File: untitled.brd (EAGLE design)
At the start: 100 x 60 mm, 43 parts, among them J1 61300311121, Q1 FQPF10N60C, Q2 s8550, Q3 s8550, T1 S8050, T2 s8050, T3 s8050

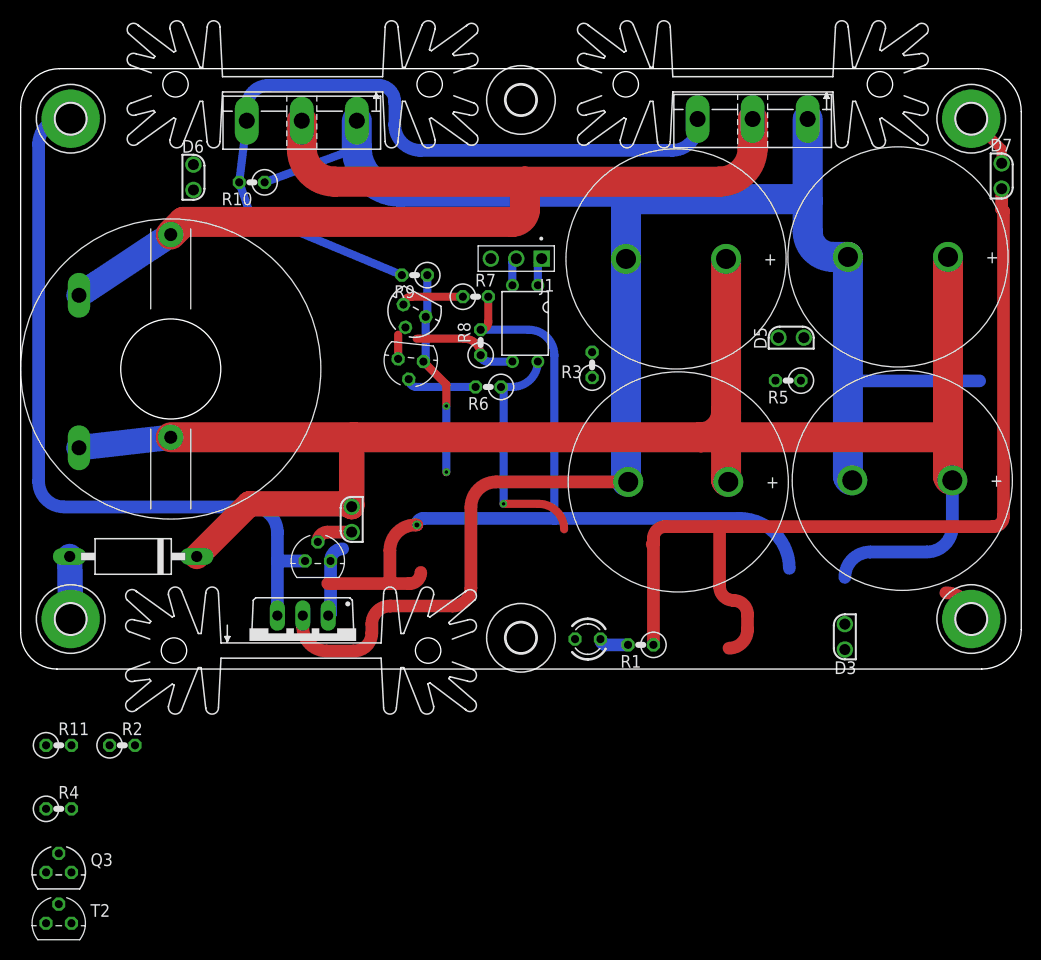
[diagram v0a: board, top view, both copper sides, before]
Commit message: add
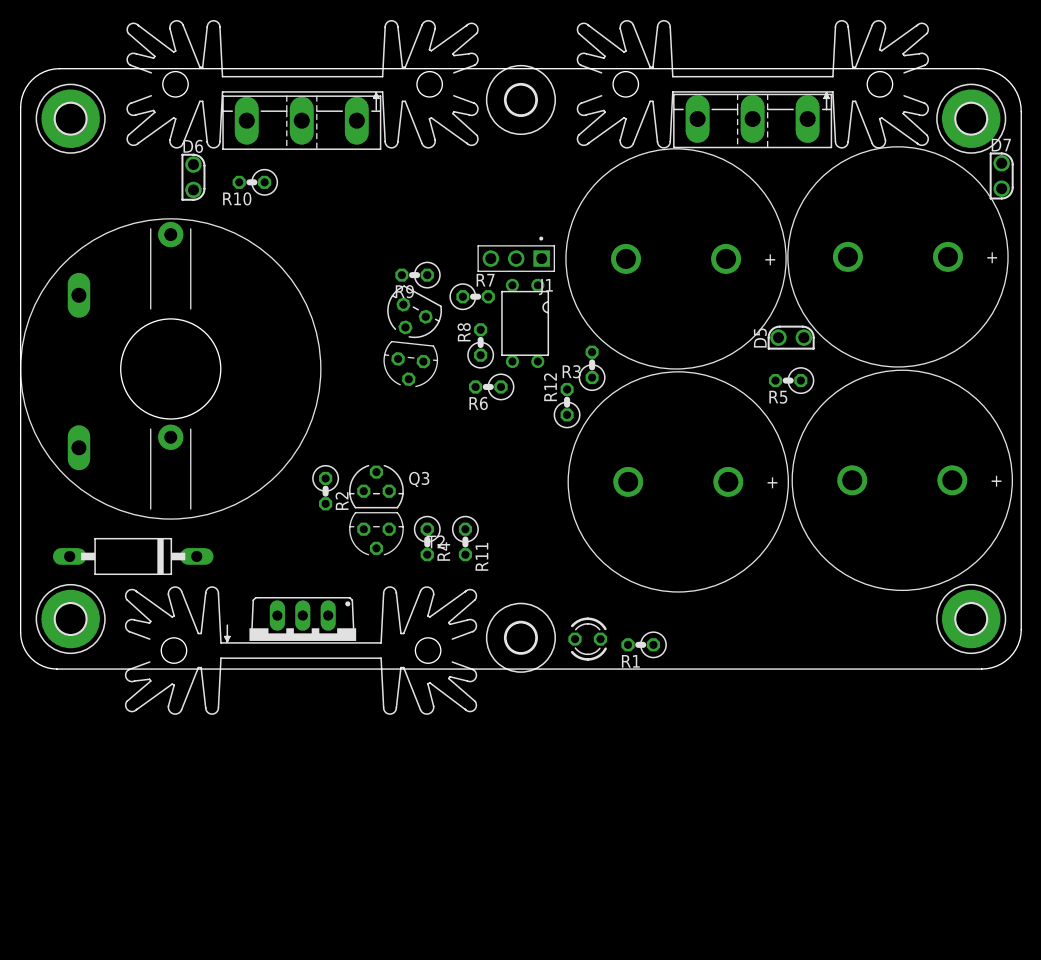
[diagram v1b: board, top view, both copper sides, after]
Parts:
- removed D3: 400v, zetex:E2LINE
- removed D4: (no value), zetex:E2LINE
- removed T1: S8050, transistor:TO92
- added R12: 37k, rcl:0207/2V
- D5: value (none) -> 440v
- R3: value 10k -> 3k
- moved T2 50.6 mm to (35.6, 14.0), turned to 180 degrees
- moved Q3 49.6 mm to (35.6, 17.8)
- moved R4 45.5 mm to (40.6, 12.7), turned to 270 degrees
- moved R11 45.4 mm to (44.5, 12.7), turned to 270 degrees
- moved R2 32.5 mm to (30.5, 17.8), turned to 270 degrees
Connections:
- new net CVO: R12.1, R3.1
- net BT-: no longer T1.3
- net CHARGE: no longer T1.1
- net N$1: now also R11.1; no longer D4.2, T1.2
- net N$10: now also R3.2; no longer R3.1
- net N$7: no longer D3.2, R11.1
- net UC: now also R12.2; no longer D3.1, D4.1, R3.2
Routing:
- net N$10: track 187.1 -> 0.00 mm
- net UC: track 179.2 -> 0.00 mm
- net BT+: track 117.2 -> 0.00 mm, vias 1 -> 0
- net N$4: track 103.7 -> 0.00 mm
- net V-: track 84.8 -> 0.00 mm, vias 1 -> 0
- net BT-: track 81.5 -> 0.00 mm
- net SWITCH: track 78.8 -> 0.00 mm
- net STOPC: track 20.8 -> 0.00 mm, vias 2 -> 0
- net N$12: track 12.9 -> 0.00 mm
- net CHARGE: track 7.27 -> 0.00 mm
- net N$14: track 7.00 -> 0.00 mm
- net N$13: track 6.27 -> 0.00 mm
- net V+: track 6.25 -> 0.00 mm
- net N$2: track 5.71 -> 0.00 mm
- net N$1: track 3.79 -> 0.00 mm
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
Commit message: add
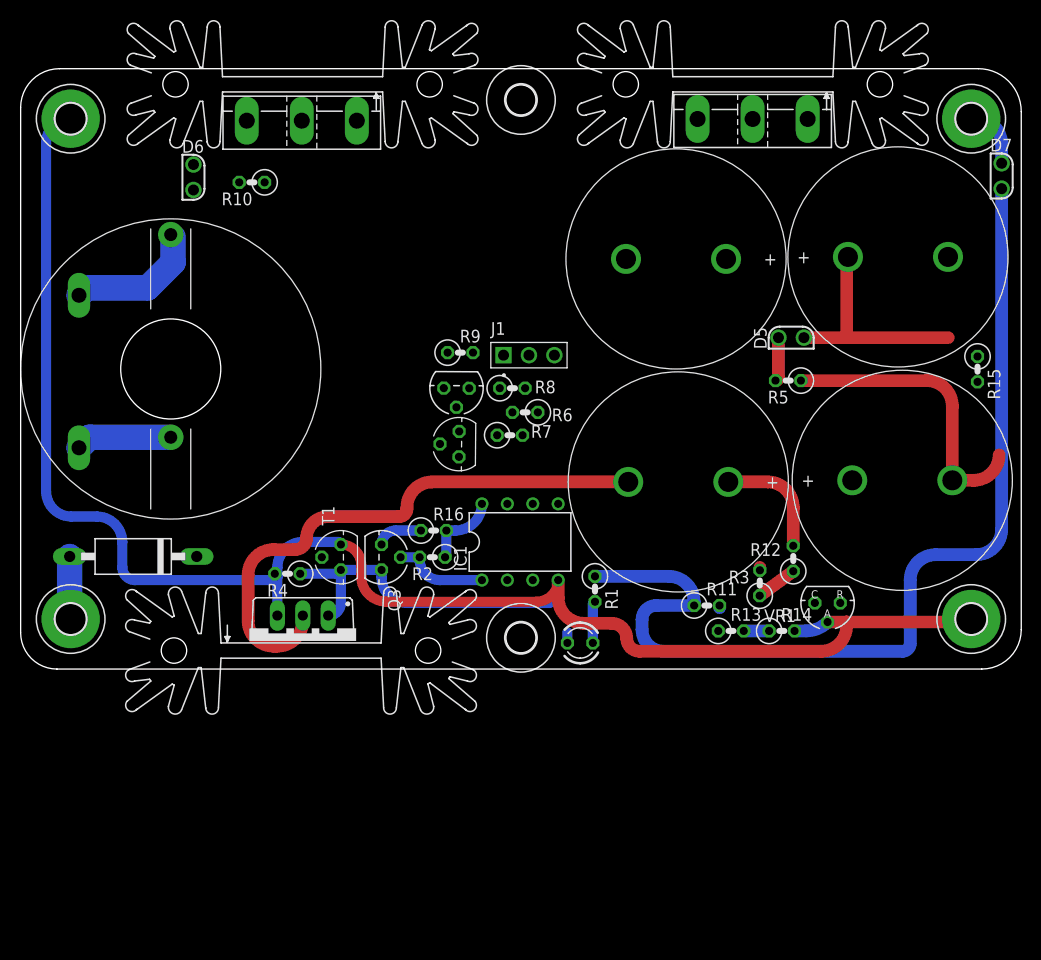
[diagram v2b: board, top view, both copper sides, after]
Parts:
- removed OK2: SFH618A-3, optocoupler:DIP4
- removed T2: s8050, transistor:TO92
- added IC1: LM393N, linear:DIL08
- added R13: 5.1k, rcl:0207/2V
- added R14: 2k, rcl:0207/2V
- added R15: 100k, rcl:0207/2V
- added R16: 1k, rcl:0207/2V
- added T1: s8050, transistor:TO92
- added VR1: (no value), v-reg:TO92-CLP
- R11: value 10k -> 470
- R12: value 37k -> 220k
- R3: value 3k -> 5.1k
- R5: value 2R -> 10R
- moved R3 27.5 mm to (73.9, 8.60), turned to 89.6 degrees
- moved R12 27.5 mm to (77.2, 11.0)
- moved R11 25.0 mm to (68.6, 6.35), turned to 0 degrees
- moved R4 14.3 mm to (26.7, 9.53), turned to 180 degrees
- moved R7 14.3 mm to (48.9, 23.4)
- moved R2 12.5 mm to (41.1, 11.2), turned to 180 degrees
- moved J1 9.74 mm to (50.8, 31.4), turned to 0 degrees
- moved T3 9.67 mm to (43.8, 22.5), turned to 89.5 degrees
- moved R9 9.00 mm to (43.9, 31.6), turned to 0 degrees
- moved Q2 8.81 mm to (43.6, 28.1), turned to 179.7 degrees
- moved R1 7.21 mm to (57.4, 8.00), turned to 270 degrees
- moved Q3 6.62 mm to (36.1, 11.2), turned to 270 degrees
- moved R8 5.57 mm to (49.1, 28.1), turned to 0 degrees
- moved R6 4.47 mm to (50.4, 25.7)
- moved LED1 0.85 mm to (55.9, 2.61)
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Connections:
- removed net N$14: R6.2, T3.2
- removed net N$9: Q3.3, R2.2
- removed net V-: R7.2, R8.2
- new net CIN: J1.1, Q2.2, R8.1, T3.1
- new net N$5: IC1.2, R11.2, R13.1, VR1.C
- net BT+: now also IC1.8, R11.1, R16.2; no longer OK2.4
- net BT-: now also IC1.4, R14.2, R7.2, R8.2, T1.1, VR1.A; no longer OK2.2, R11.2
- net CHARGE: now also R4.1, T1.3; no longer T2.2
- net CVO: now also IC1.3
- net N$1: now also IC1.1, Q3.2, R2.2; no longer R11.1
- net N$10: now also Q3.3, R16.1; no longer D6.2, Q1.D, R10.1, R3.2, R5.1, U$1.-, U$13.E, U$2.-, U$3.-, U$4.-, U$9.E
- net N$11: now also Q2.3, R6.2; no longer J1.1, OK2.1
- net N$12: now also Q2.1, R9.1, T3.2; no longer OK2.3, Q2.2, R8.1, T3.1
- net N$13: now also T3.3; no longer Q2.1
- net N$7: now also R13.2, R14.1, VR1.R; no longer Q3.2, T2.1
- net N$8: now also D6.2, Q1.D, R10.1, R15.2, R3.2, R5.1, U$1.-, U$13.E, U$2.-, U$3.-, U$4.-, U$9.E; no longer R4.1, T2.3
- net STOPC: now also T1.2; no longer Q2.3, R9.1, T3.3
- net UC: now also R15.1
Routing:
- net BT-: track 0.00 -> 157.1 mm
- net BT+: track 0.00 -> 105.2 mm
- net N$8: track 0.00 -> 84.2 mm
- net UC: track 0.00 -> 43.6 mm
- net CHARGE: track 0.00 -> 33.2 mm
- net N$4: track 0.00 -> 13.3 mm
- net N$1: track 0.00 -> 9.22 mm
- net V+: track 0.00 -> 6.55 mm
- net N$2: track 0.00 -> 6.01 mm
- net N$10: track 0.00 -> 4.52 mm
- net N$3: track 0.00 -> 4.41 mm
- net N$6: track 0.00 -> 4.20 mm
- net CVO: track 0.00 -> 4.15 mm
- net N$7: track 0.00 -> 2.54 mm
